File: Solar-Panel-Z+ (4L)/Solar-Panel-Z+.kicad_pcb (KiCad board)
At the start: 4 copper layers, 48.4 x 48.4 mm, 79 parts, among them J1 FTS-105-01-X-DV-A, Q1 NX3008NBKS, Q2 MBT2222ADW1T1, Q3 NX3008NBKS, Q4 MBT2222ADW1T1, U1 BQ25570RGRR, U2 OPT3001, U3 MAX40200AUK

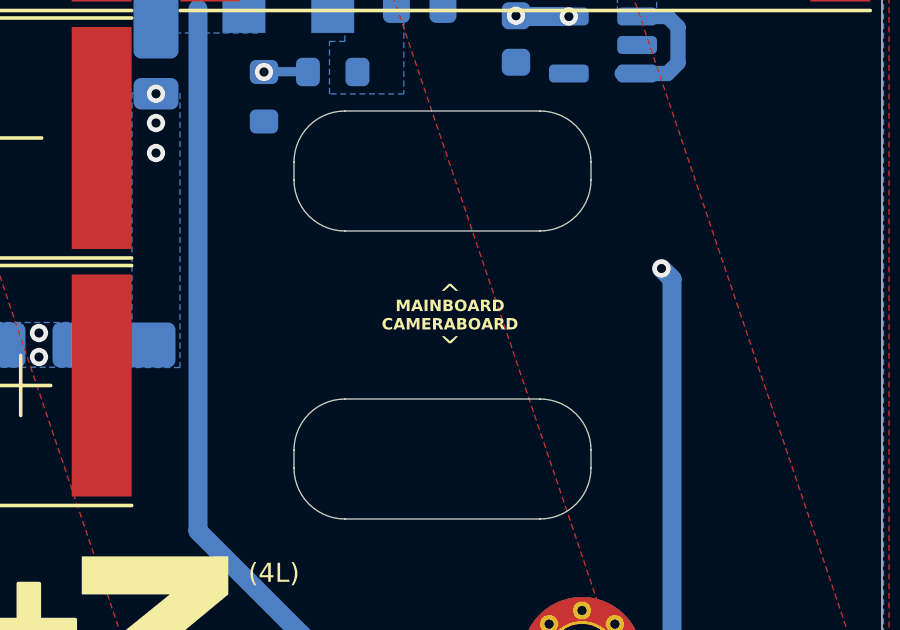
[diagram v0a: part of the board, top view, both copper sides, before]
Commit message: B3/02 Updates
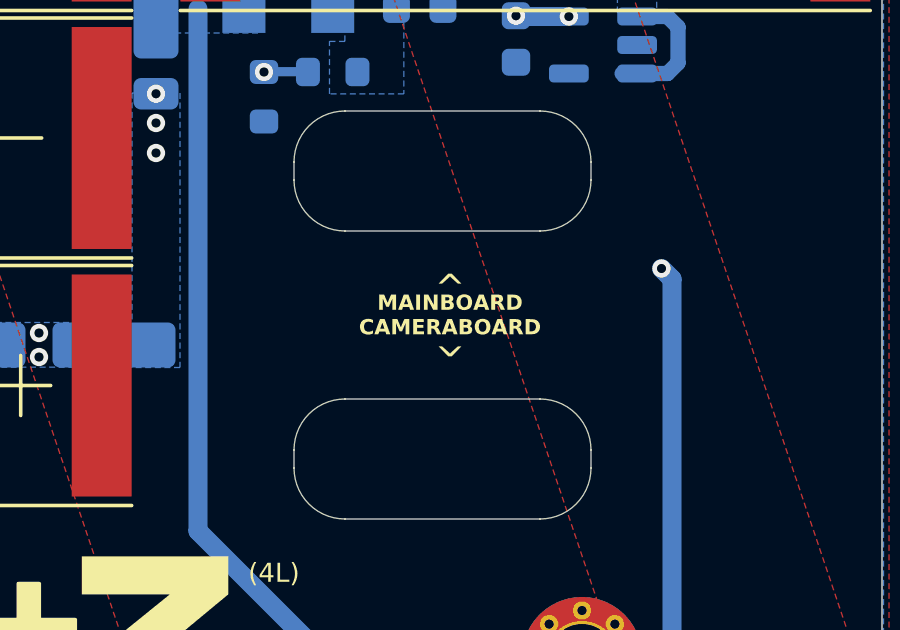
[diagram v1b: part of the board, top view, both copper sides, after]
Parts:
- C1: value 1uF -> 0.1uF
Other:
- board text added: "Rev B3/02"
- board text removed: "Rev B3/01"
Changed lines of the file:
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@@
     (39 "F.Mask" user)
     (40 "Dwgs.User" user "User.Drawings")
-    (41 "Cmts.User" user "User.Comments")
     (44 "Edge.Cuts" user)
     (45 "Margin" user)
@@
         (effects (font (size 0.381 0.381) (thickness 0.0762)))
     )
-    (fp_text value "1uF" (at 0 1.17 90) (layer "F.Fab")
+    (fp_text value "0.1uF" (at 0 1.17 90) (layer "F.Fab")
         (effects (font (size 1 1) (thickness 0.15)))
     )
@@
     (descr "Circular Fiducial, 0.75mm bare copper, 1.5mm soldermask opening (Level B)")
     (tags "fiducial")
-    (attr smd)
+    (attr smd exclude_from_bom)
     (fp_text reference "REF**" (at 0 -2) (layer "F.SilkS") hide
         (effects (font (size 1 1) (thickness 0.15)))
@@
     (property "Sheetfile" "Solar-Panel-Z+.kicad_sch")
     (property "Sheetname" "")
+    (property "exclude_from_bom" "")
     (property "ki_description" "Mounting Hole with connection")
     (property "ki_keywords" "mounting hole")
@@
     (fp_circle (center 0 0) (end 2.15 0)
       (stroke (width 0.05) (type solid)) (fill none) (layer "F.CrtYd"))
-    (pad "" np_thru_hole circle (at 0 0) (size 2.4 2.4) (drill 2.2) (layers "F&B.Cu" "*.Mask"))
+    (pad "" np_thru_hole circle (at 0 0) (size 2.4 2.4) (drill 2.2) (layers "*.Cu" "*.Mask"))
     (pad "1" thru_hole circle (at -1.55 0) (size 0.6096 0.6096) (drill 0.3048) (layers "*.Cu" "*.Mask")
       (net 1 "GND") (pinfunction "1") (pintype "input"))
@@
     (descr "Circular Fiducial, 0.75mm bare copper, 1.5mm soldermask opening (Level B)")
     (tags "fiducial")
-    (attr smd)
+    (attr smd exclude_from_bom)
     (fp_text reference "REF**" (at 0 -2) (layer "F.SilkS") hide
         (effects (font (size 1 1) (thickness 0.15)))
@@
     (descr "Circular Fiducial, 0.75mm bare copper, 1.5mm soldermask opening (Level B)")
     (tags "fiducial")
-    (attr smd)
+    (attr smd exclude_from_bom)
     (fp_text reference "REF**" (at 0 -2) (layer "F.SilkS") hide
         (effects (font (size 1 1) (thickness 0.15)))
@@
     (property "Sheetfile" "Solar-Panel-Z+.kicad_sch")
     (property "Sheetname" "")
+    (property "exclude_from_bom" "")
     (property "ki_description" "Mounting Hole with connection")
     (property "ki_keywords" "mounting hole")
@@
     (fp_circle (center 0 0) (end 2.15 0)
       (stroke (width 0.05) (type solid)) (fill none) (layer "F.CrtYd"))
-    (pad "" np_thru_hole circle (at 0 0) (size 2.4 2.4) (drill 2.2) (layers "F&B.Cu" "*.Mask"))
+    (pad "" np_thru_hole circle (at 0 0) (size 2.4 2.4) (drill 2.2) (layers "*.Cu" "*.Mask"))
     (pad "1" thru_hole circle (at -1.55 0) (size 0.6096 0.6096) (drill 0.3048) (layers "*.Cu" "*.Mask")
       (net 1 "GND") (pinfunction "1") (pintype "input"))
@@
   (footprint "custom-footprints:ypanel" (layer "F.Cu")
     (at 106.010401 86.552858)
-    (attr through_hole)
+    (attr through_hole exclude_from_bom)
     (fp_text reference "Ref**" (at -3.15 0.19) (layer "F.SilkS") hide
         (effects (font (size 1.27 1.27) (thickness 0.15)))
@@
     (property "Sheetfile" "Solar-Panel-Z+.kicad_sch")
     (property "Sheetname" "")
+    (property "exclude_from_bom" "")
     (property "ki_description" "Mounting Hole with connection")
     (property "ki_keywords" "mounting hole")
@@
     (fp_circle (center 0 0) (end 2.15 0)
       (stroke (width 0.05) (type solid)) (fill none) (layer "F.CrtYd"))
-    (pad "" np_thru_hole circle (at 0 0) (size 2.4 2.4) (drill 2.2) (layers "F&B.Cu" "*.Mask"))
+    (pad "" np_thru_hole circle (at 0 0) (size 2.4 2.4) (drill 2.2) (layers "*.Cu" "*.Mask"))
     (pad "1" thru_hole circle (at -1.55 0) (size 0.6096 0.6096) (drill 0.3048) (layers "*.Cu" "*.Mask")
       (net 1 "GND") (pinfunction "1") (pintype "input"))
@@
     (property "Sheetfile" "Solar-Panel-Z+.kicad_sch")
     (property "Sheetname" "")
+    (property "exclude_from_bom" "")
     (property "ki_description" "Mounting Hole with connection")
     (property "ki_keywords" "mounting hole")
@@
     (fp_circle (center 0 0) (end 2.15 0)
       (stroke (width 0.05) (type solid)) (fill none) (layer "F.CrtYd"))
-    (pad "" np_thru_hole circle (at 0 0) (size 2.4 2.4) (drill 2.2) (layers "F&B.Cu" "*.Mask"))
+    (pad "" np_thru_hole circle (at 0 0) (size 2.4 2.4) (drill 2.2) (layers "*.Cu" "*.Mask"))
     (pad "1" thru_hole circle (at -1.55 0) (size 0.6096 0.6096) (drill 0.3048) (layers "*.Cu" "*.Mask")
       (net 1 "GND") (pinfunction "1") (pintype "input"))
@@
     (property "Sheetfile" "Solar-Panel-Z+.kicad_sch")
     (property "Sheetname" "")
+    (property "exclude_from_bom" "")
     (property "ki_description" "test point")
     (property "ki_keywords" "test point tp")
-    (attr exclude_from_pos_files)
+    (attr exclude_from_pos_files exclude_from_bom)
     (fp_text reference "TP2" (at 0 1.448) (layer "B.SilkS") hide
         (effects (font (size 1 1) (thickness 0.15)) (justify mirror))
@@
     (property "Sheetfile" "Solar-Panel-Z+.kicad_sch")
     (property "Sheetname" "")
+    (property "exclude_from_bom" "")
     (property "ki_description" "test point")
     (property "ki_keywords" "test point tp")
-    (attr exclude_from_pos_files)
+    (attr exclude_from_pos_files exclude_from_bom)
     (fp_text reference "TP3" (at 0 1.448) (layer "B.SilkS") hide
         (effects (font (size 1 1) (thickness 0.15)) (justify mirror))
@@
     (property "Sheetfile" "Solar-Panel-Z+.kicad_sch")
     (property "Sheetname" "")
+    (property "exclude_from_bom" "")
     (property "ki_description" "test point")
     (property "ki_keywords" "test point tp")
-    (attr exclude_from_pos_files)
+    (attr exclude_from_pos_files exclude_from_bom)
     (fp_text reference "TP4" (at 0 1.448) (layer "B.SilkS") hide
         (effects (font (size 1 1) (thickness 0.15)) (justify mirror))
@@
     (property "Sheetfile" "Solar-Panel-Z+.kicad_sch")
     (property "Sheetname" "")
+    (property "exclude_from_bom" "")
     (property "ki_description" "test point")
     (property "ki_keywords" "test point tp")
-    (attr exclude_from_pos_files)
+    (attr exclude_from_pos_files exclude_from_bom)
     (fp_text reference "TP1" (at 0 1.448) (layer "B.SilkS") hide
         (effects (font (size 1 1) (thickness 0.15)) (justify mirror))
@@
     (descr "Circular Fiducial, 0.75mm bare copper, 1.5mm soldermask opening (Level B)")
     (tags "fiducial")
-    (attr smd)
+    (attr smd exclude_from_bom)
     (fp_text reference "REF**" (at 0 2) (layer "B.SilkS") hide
         (effects (font (size 1 1) (thickness 0.15)) (justify mirror))
@@
     (descr "Circular Fiducial, 0.75mm bare copper, 1.5mm soldermask opening (Level B)")
     (tags "fiducial")
-    (attr smd)
+    (attr smd exclude_from_bom)
     (fp_text reference "REF**" (at 0 2) (layer "B.SilkS") hide
         (effects (font (size 1 1) (thickness 0.15)) (justify mirror))
@@
     (descr "Circular Fiducial, 0.75mm bare copper, 1.5mm soldermask opening (Level B)")
     (tags "fiducial")
-    (attr smd)
+    (attr smd exclude_from_bom)
     (fp_text reference "REF**" (at 0 2) (layer "B.SilkS") hide
         (effects (font (size 1 1) (thickness 0.15)) (justify mirror))
@@
   (footprint "custom-footprints:pycubed_mini_half" (layer "B.Cu")
     (at 106.2 44.5 180)
-    (attr through_hole)
+    (attr through_hole exclude_from_bom)
     (fp_text reference "Ref**" (at 0 0) (layer "B.SilkS") hide
         (effects (font (size 1.27 1.27) (thickness 0.15)) (justify mirror))
@@
     (effects (font (size 0.508 0.508) (thickness 0.1016)))
   )
-  (gr_text "^" (at 116.5 76.9 180) (layer "F.SilkS")
-    (effects (font (size 0.635 0.635) (thickness 0.1016)))
+  (gr_text "^" (at 116.5 77.2 180) (layer "F.SilkS")
+    (effects (font (size 0.889 0.889) (thickness 0.127)))
   )
   (gr_text "MAINBOARD\nCAMERABOARD" (at 116.5 76.3) (layer "F.SilkS")
-    (effects (font (size 0.381 0.381) (thickness 0.0762) bold))
+    (effects (font (size 0.508 0.508) (thickness 0.1016) bold))
   )
   (gr_text "-" (at 109.1 43.5 90) (layer "F.SilkS")
@@
     (effects (font (size 0.508 0.508) (thickness 0.1016)))
   )
-  (gr_text "^" (at 116.5 75.6) (layer "F.SilkS")
-    (effects (font (size 0.635 0.635) (thickness 0.1016)))
+  (gr_text "^" (at 116.5 75.4) (layer "F.SilkS")
+    (effects (font (size 0.889 0.889) (thickness 0.127)))
   )
   (gr_text "S" (at 117.9 88.05) (layer "F.SilkS")
@@
     (effects (font (size 0.635 0.635) (thickness 0.127)))
   )
-  (gr_text "Rev B3/01" (at 105.825 46.665) (layer "B.Mask")
+  (gr_text "Rev B3/02" (at 105.825 46.665) (layer "B.Mask")
     (effects (font (size 0.635 0.635) (thickness 0.1524)) (justify mirror))
   )
